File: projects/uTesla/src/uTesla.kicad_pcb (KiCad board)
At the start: 2 copper layers, 140 x 140 mm, 75 parts, among them J1 DC-005, J2 Flash, J3 IO, J4 MSD-1-A, Q1 IRFZ44N, Q2 IRFZ44N, Q3 IRFZ44N, SW1 RST, T1 1:1, U1 MP9486A, U2 AMS1117-3.3, U3 ATmega328P-A, Y1 HC-49 16MHz

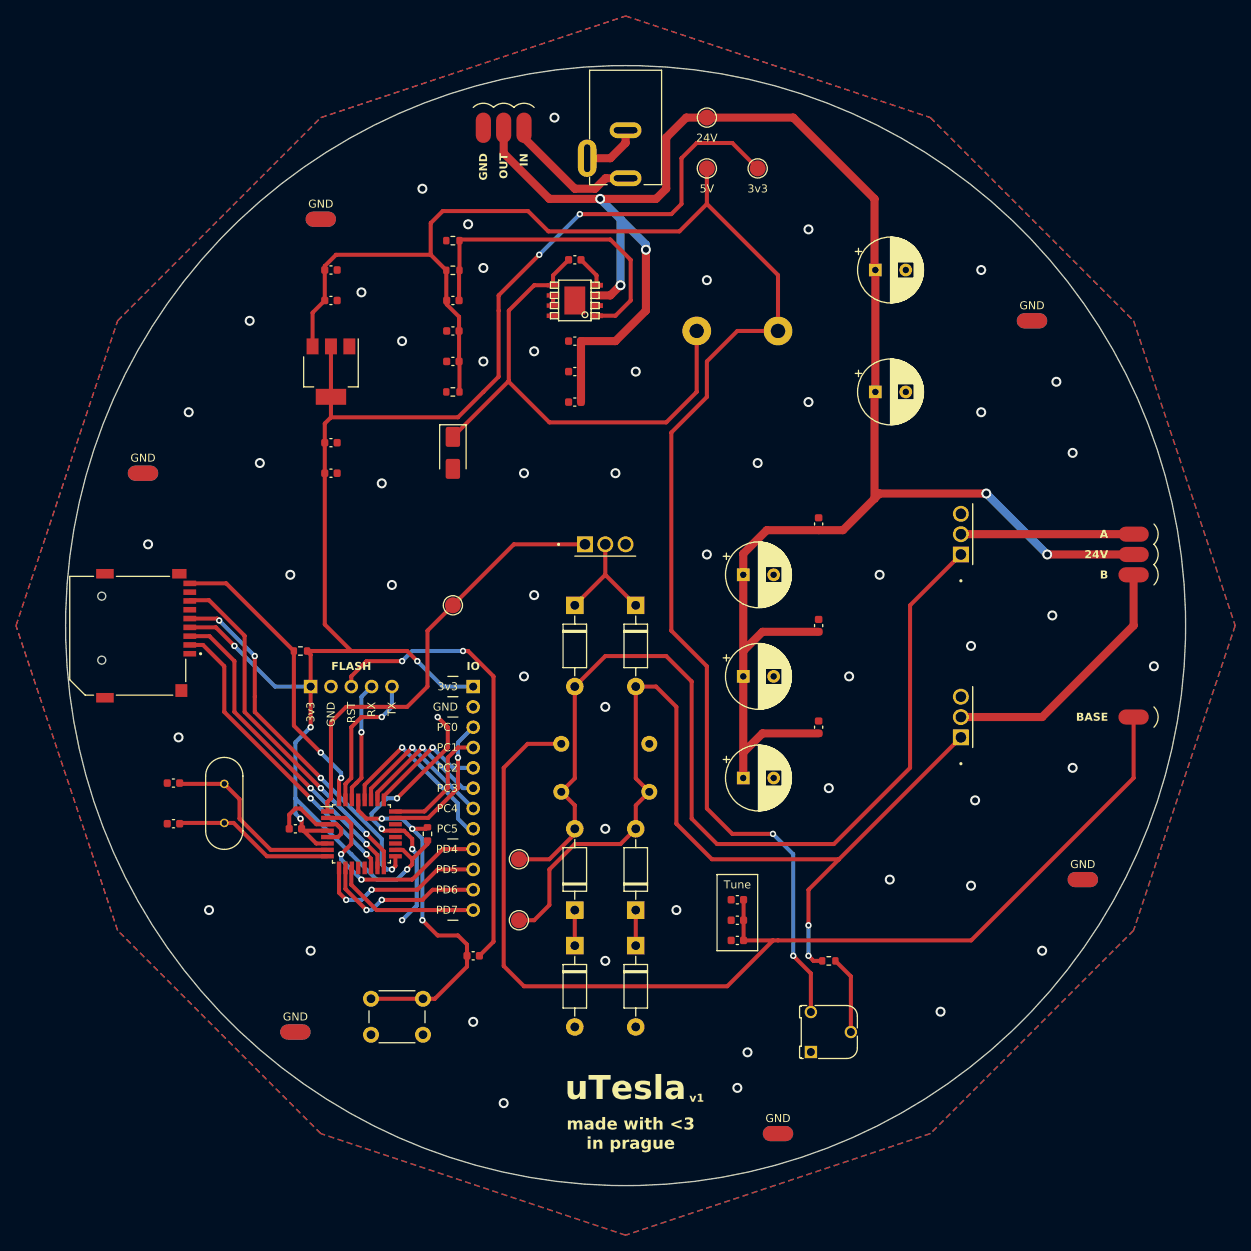
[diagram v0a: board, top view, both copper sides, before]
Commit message: Update source files
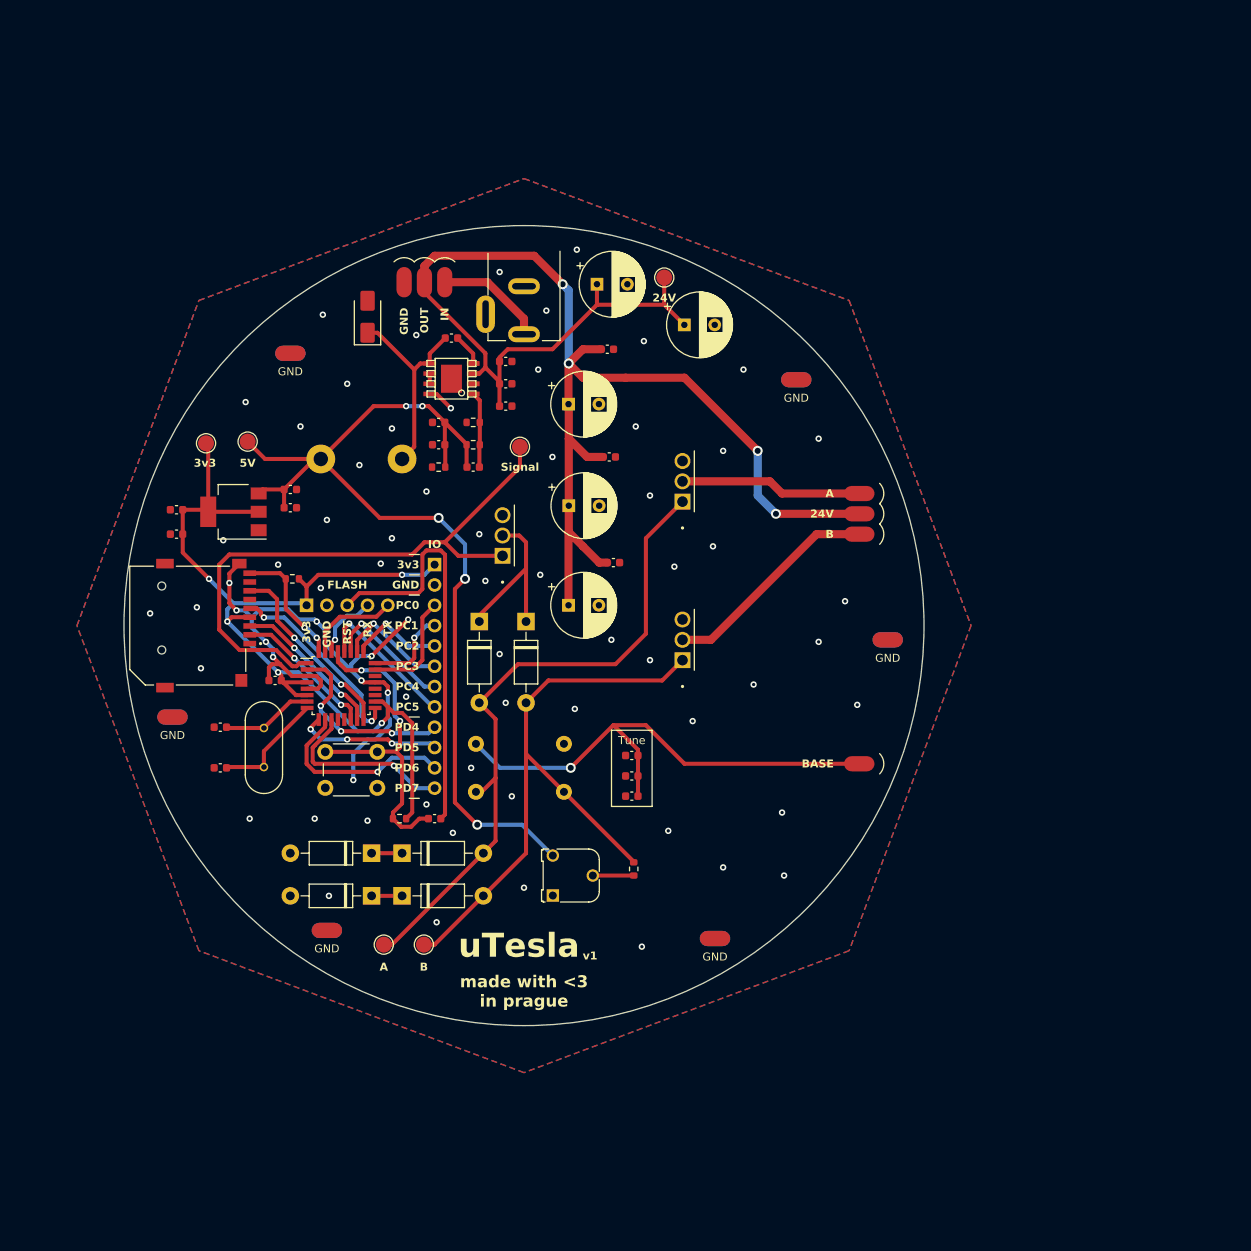
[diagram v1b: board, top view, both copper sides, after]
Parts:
- moved TP3 77.0 mm to (100.0, 66.1)
- moved TP2 66.8 mm to (105.2, 65.9)
- moved L1 40.2 mm to (124.5, 68.1), turned to -90 degrees
- moved J11 38.6 mm to (185.2, 90.7)
- moved J17 38.6 mm to (185.2, 90.7)
- moved RV1 37.7 mm to (143.3, 122.6)
- moved Q3 36.1 mm to (159.5, 90.7)
- moved Q2 35.4 mm to (159.5, 70.9)
- moved C1 34.8 mm to (148.8, 46.2)
- moved J6 34.8 mm to (181.6, 106.2)
- moved J5 34.7 mm to (181.6, 74.9)
- moved C21 34.3 mm to (150.1, 54.4), turned to 0 degrees
- moved C22 33.6 mm to (150.4, 67.8), turned to 0 degrees
- moved D7 33.6 mm to (120.7, 122.7), turned to 180 degrees
- moved C23 32.9 mm to (150.9, 81.0), turned to 0 degrees
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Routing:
- net +3V3: track 215.5 -> 122.6 mm, vias 7 -> 5
- net +5V: track 212.5 -> 123.5 mm, vias 2 -> 5
- net /Contacts/Base: track 140.2 -> 63.5 mm, vias 0 -> 1
- net +24V: track 251.0 -> 183.9 mm, vias 5 -> 4
- net Net-(D3-A): track 121.2 -> 77.2 mm, vias 2 -> 0
- net Net-(D2-A): track 124.6 -> 83.4 mm
- net Net-(D1-K): track 64.4 -> 25.8 mm
- net Net-(U1-FB): track 40.1 -> 9.51 mm
- net GND: track 54.5 -> 78.3 mm, vias 57 -> 70
- net /Microcontroller/Card: track 37.7 -> 15.7 mm
- net /Microcontroller/SCK: track 46.0 -> 24.6 mm, vias 4 -> 2
- net /Microcontroller/MISO: track 45.0 -> 23.7 mm
- net /Microcontroller/MOSI: track 40.1 -> 19.2 mm
- net /Microcontroller/CS: track 38.2 -> 17.8 mm
- net /Driver/Signal: track 56.4 -> 74.3 mm
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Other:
- board size 140 x 140 mm -> 100 x 100 mm
- board text added: "Signal"
